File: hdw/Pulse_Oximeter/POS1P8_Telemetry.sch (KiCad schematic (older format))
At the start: 11 parts, among them U701 INA219BxDCN, U702 MCP9804, U703 INA219BxDCN

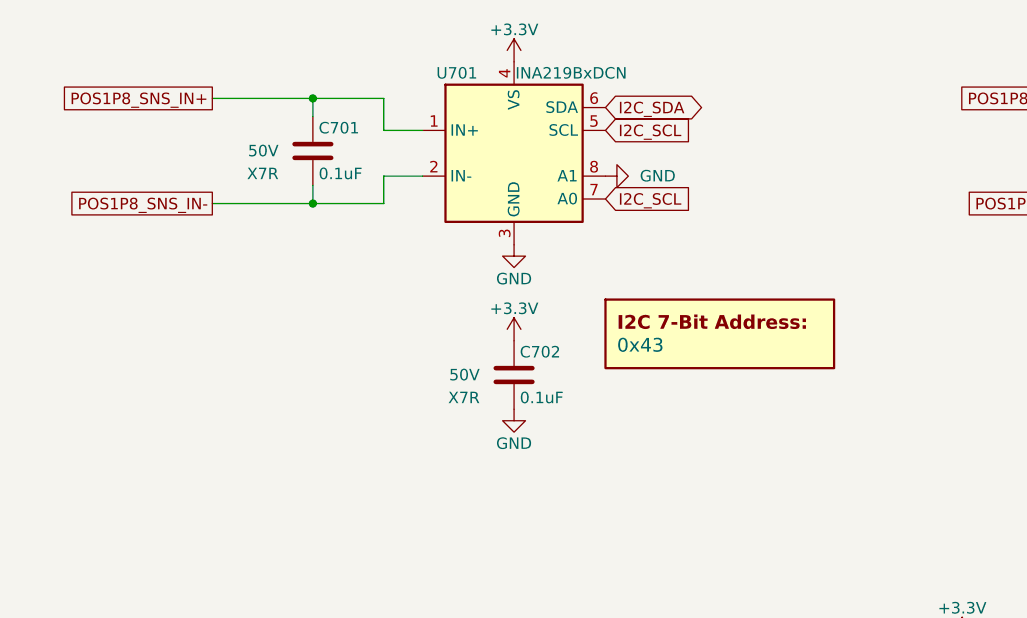
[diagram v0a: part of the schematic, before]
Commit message: More part arrangements
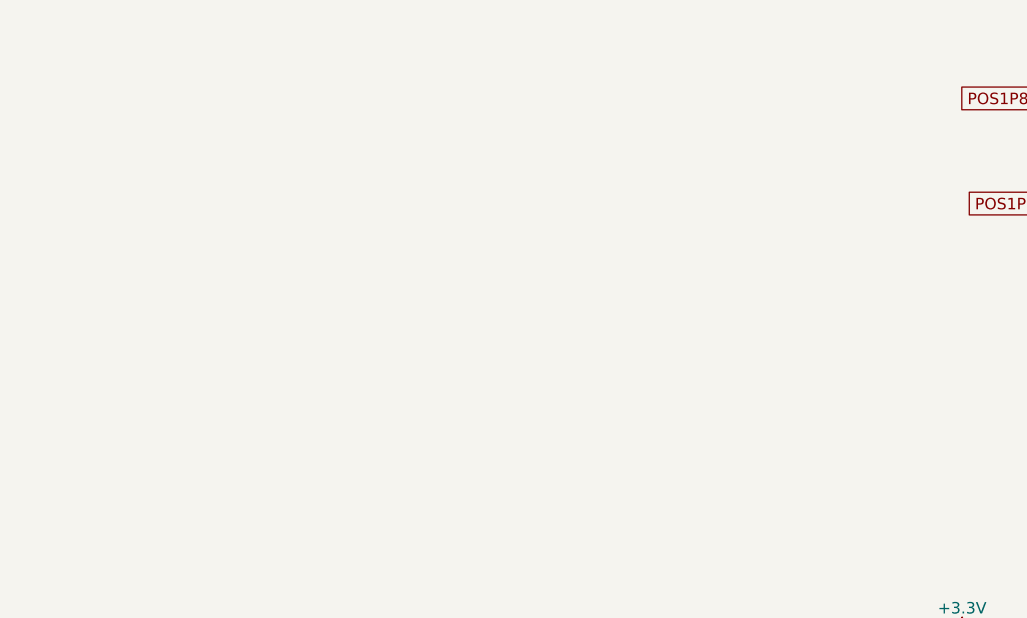
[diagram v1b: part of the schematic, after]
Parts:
- removed C701, C702: 0.1uF, Capacitors_SMD:C_0402, symbol Custom_Library:C_Custom
- removed DOC701: 0x43, symbol Custom_Library:I2C_Address
- removed U701: INA219BxDCN, Package_TO_SOT_SMD:SOT-23-8, symbol Analog_ADC:INA219BxDCN
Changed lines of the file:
@@
 $Descr A 11000 8500
 encoding utf-8
-Sheet 7 23
+Sheet 7 21
 Title "Pulse Oximeter"
 Date "2019-01-03"
@@
 Comment4 ""
 $EndDescr
-Text GLabel 2150 1970 0    50   UnSpc ~ 0
-POS1P8_SNS_IN+
-Text GLabel 2150 2430 0    50   UnSpc ~ 0
-POS1P8_SNS_IN-
 $Comp
 L power:GND #PWR?
@@
 $Comp
 L power:GND #PWR?
-U 1 1 5EC52D0D
-P 3470 2610
-AR Path="/5E0652BA/5EC52D0D" Ref="#PWR?"  Part="1"
-AR Path="/5E0A0E29/5EC52D0D" Ref="#PWR?"  Part="1"
-AR Path="/5E052856/5EC52D0D" Ref="#PWR?"  Part="1"
-AR Path="/5EAE2E6F/5EC52D0D" Ref="#PWR0702"  Part="1"
-F 0 "#PWR0702" H 3470 2360 50  0001 C CNN
-F 1 "GND" H 3470 2460 50  0000 C CNN
-F 2 "" H 3470 2610 50  0001 C CNN
-F 3 "" H 3470 2610 50  0001 C CNN
-	1    3470 2610
-	1    0    0    -1
-$EndComp
-$Comp
-L power:+3.3V #PWR?
-U 1 1 5E1BD4C4
-P 3470 1810
-AR Path="/5E0652BA/5E1BD4C4" Ref="#PWR?"  Part="1"
-AR Path="/5E0A0E29/5E1BD4C4" Ref="#PWR?"  Part="1"
-AR Path="/5E052856/5E1BD4C4" Ref="#PWR?"  Part="1"
-AR Path="/5EAE2E6F/5E1BD4C4" Ref="#PWR0701"  Part="1"
-F 0 "#PWR0701" H 3470 1660 50  0001 C CNN
-F 1 "+3.3V" H 3470 1950 50  0000 C CNN
-F 2 "" H 3470 1810 50  0001 C CNN
-F 3 "" H 3470 1810 50  0001 C CNN
-	1    3470 1810
-	1    0    0    -1
-$EndComp
-Text GLabel 3870 2110 2    50   Input ~ 0
-I2C_SCL
-$Comp
-L Custom_Library:C_Custom C?
-U 1 1 5E1BD4CF
-P 3470 3180
-AR Path="/5B3E071A/5E1BD4CF" Ref="C?"  Part="1"
-AR Path="/5E0652BA/5E1BD4CF" Ref="C?"  Part="1"
-AR Path="/5E0A0E29/5E1BD4CF" Ref="C?"  Part="1"
-AR Path="/5E052856/5E1BD4CF" Ref="C?"  Part="1"
-AR Path="/5EAE2E6F/5E1BD4CF" Ref="C702"  Part="1"
-F 0 "C702" H 3495 3280 50  0000 L CNN
-F 1 "0.1uF" H 3495 3080 50  0000 L CNN
-F 2 "Capacitors_SMD:C_0402" H 3508 3030 50  0001 C CNN
-F 3 "" H 3495 3280 50  0001 C CNN
-F 4 "" H 3320 3280 50  0000 R CNN "display_footprint"
-F 5 "50V" H 3320 3180 50  0000 R CNN "Voltage"
-F 6 "X7R" H 3320 3080 50  0000 R CNN "Dielectric"
-F 7 "490-10701-1-ND" H -440 -3700 50  0001 C CNN "Digi-Key PN"
-	1    3470 3180
-	1    0    0    -1
-$EndComp
-$Comp
-L power:+3.3V #PWR?
-U 1 1 5E1BD4D5
-P 3470 3030
-AR Path="/5E0652BA/5E1BD4D5" Ref="#PWR?"  Part="1"
-AR Path="/5E0A0E29/5E1BD4D5" Ref="#PWR?"  Part="1"
-AR Path="/5E052856/5E1BD4D5" Ref="#PWR?"  Part="1"
-AR Path="/5EAE2E6F/5E1BD4D5" Ref="#PWR0703"  Part="1"
-F 0 "#PWR0703" H 3470 2880 50  0001 C CNN
-F 1 "+3.3V" H 3470 3170 50  0000 C CNN
-F 2 "" H 3470 3030 50  0001 C CNN
-F 3 "" H 3470 3030 50  0001 C CNN
-	1    3470 3030
-	1    0    0    -1
-$EndComp
-$Comp
-L power:GND #PWR?
-U 1 1 5E1BD4DB
-P 3470 3330
-AR Path="/5E0652BA/5E1BD4DB" Ref="#PWR?"  Part="1"
-AR Path="/5E0A0E29/5E1BD4DB" Ref="#PWR?"  Part="1"
-AR Path="/5E052856/5E1BD4DB" Ref="#PWR?"  Part="1"
-AR Path="/5EAE2E6F/5E1BD4DB" Ref="#PWR0704"  Part="1"
-F 0 "#PWR0704" H 3470 3080 50  0001 C CNN
-F 1 "GND" H 3470 3180 50  0000 C CNN
-F 2 "" H 3470 3330 50  0001 C CNN
-F 3 "" H 3470 3330 50  0001 C CNN
-	1    3470 3330
-	1    0    0    -1
-$EndComp
-Text GLabel 3870 2010 2    50   BiDi ~ 0
-I2C_SDA
-Wire Wire Line
-	2590 2430 2590 2350
-Wire Wire Line
-	2590 2050 2590 1970
-$Comp
-L Custom_Library:C_Custom C?
-U 1 1 5E1BD4F9
-P 2590 2200
-AR Path="/5B3E071A/5E1BD4F9" Ref="C?"  Part="1"
-AR Path="/5E0652BA/5E1BD4F9" Ref="C?"  Part="1"
-AR Path="/5E0A0E29/5E1BD4F9" Ref="C?"  Part="1"
-AR Path="/5E052856/5E1BD4F9" Ref="C?"  Part="1"
-AR Path="/5EAE2E6F/5E1BD4F9" Ref="C701"  Part="1"
-F 0 "C701" H 2615 2300 50  0000 L CNN
-F 1 "0.1uF" H 2615 2100 50  0000 L CNN
-F 2 "Capacitors_SMD:C_0402" H 2628 2050 50  0001 C CNN
-F 3 "" H 2615 2300 50  0001 C CNN
-F 4 "" H 2440 2300 50  0000 R CNN "display_footprint"
-F 5 "50V" H 2440 2200 50  0000 R CNN "Voltage"
-F 6 "X7R" H 2440 2100 50  0000 R CNN "Dielectric"
-F 7 "490-10701-1-ND" H -1320 -4680 50  0001 C CNN "Digi-Key PN"
-	1    2590 2200
-	1    0    0    -1
-$EndComp
-Wire Wire Line
-	2150 2430 2590 2430
-Wire Wire Line
-	2150 1970 2590 1970
-Wire Wire Line
-	3070 2110 2900 2110
-Wire Wire Line
-	2900 2110 2900 1970
-Wire Wire Line
-	2900 1970 2590 1970
-Connection ~ 2590 1970
-Wire Wire Line
-	3070 2310 2900 2310
-Wire Wire Line
-	2900 2310 2900 2430
-Wire Wire Line
-	2900 2430 2590 2430
-Connection ~ 2590 2430
-$Comp
-L power:GND #PWR?
 U 1 1 5E1C292F
 P 7470 2610
@@
 Connection ~ 6590 2430
 $Comp
-L Analog_ADC:INA219BxDCN U701
-U 1 1 5E1BD516
-P 3470 2210
-F 0 "U701" H 3220 2560 50  0000 C CNN
-F 1 "INA219BxDCN" H 3720 2560 50  0000 C CNN
-F 2 "Package_TO_SOT_SMD:SOT-23-8" H 4120 1860 50  0001 C CNN
-F 3 "http://www.ti.com/lit/ds/symlink/ina219.pdf" H 3820 2110 50  0001 C CNN
-F 4 "296-46420-1-ND" H 3470 2210 50  0001 C CNN "Digi-Key PN"
-F 5 "Telemetry" H 3470 2210 50  0001 C CNN "Configuration"
-	1    3470 2210
-	1    0    0    -1
-$EndComp
-$Comp
 L Custom_Library:I2C_Address DOC?
-U 1 1 5EC2F63C
-P 4370 3050
-AR Path="/5E0652BA/5EC2F63C" Ref="DOC?"  Part="1"
-AR Path="/5E0A0E29/5EC2F63C" Ref="DOC?"  Part="1"
-AR Path="/5E052856/5EC2F63C" Ref="DOC?"  Part="1"
-AR Path="/5EAE2DDC/5EC2F63C" Ref="DOC?"  Part="1"
-AR Path="/5EAE2E6F/5EC2F63C" Ref="DOC701"  Part="1"
-F 0 "DOC701" H 4370 3300 60  0001 C CNN
-F 1 "0x43" H 3920 3050 60  0000 L CNN
-F 2 "" H 4370 3400 60  0001 C CNN
-F 3 "" H 4370 3400 60  0001 C CNN
-	1    4370 3050
-	1    0    0    -1
-$EndComp
-$Comp
-L power:GND #PWR?
-U 1 1 5EC2F642
-P 3870 2310
-AR Path="/5EAE2DDC/5EC2F642" Ref="#PWR?"  Part="1"
-AR Path="/5EAE2E6F/5EC2F642" Ref="#PWR0705"  Part="1"
-F 0 "#PWR0705" H 3870 2060 50  0001 C CNN
-F 1 "GND" V 3870 2160 50  0000 R CNN
-F 2 "" H 3870 2310 50  0001 C CNN
-F 3 "" H 3870 2310 50  0001 C CNN
-	1    3870 2310
-	0    -1   -1   0
-$EndComp
-Text GLabel 3870 2410 2    50   Input ~ 0
-I2C_SCL
-$Comp
-L Custom_Library:I2C_Address DOC?
